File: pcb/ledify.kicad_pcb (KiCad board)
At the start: 4 copper layers, 35.5 x 52.5 mm, 74 parts, among them J1 Conn_01x01_Pin, J2 USB_C_Receptacle_USB2.0_16P, J3 Conn_01x01_Pin, J4 Conn_01x01_Pin, Q1 2N7002K, SW1 TS-1088-AR02016, SW2 TS-1088-AR02016, U1 ESP32-C6_C5364646, U2 USBLC6-2P6, U3 AP63203WU, U4 FUSB302BMPX, U5 W25Q128JVP, U6 LM61495QRPHRQ1, U7 BMI323, U8 BMP581, X1 XL2EL89COI-111YLC-40M, X2 Q13FC1350000400

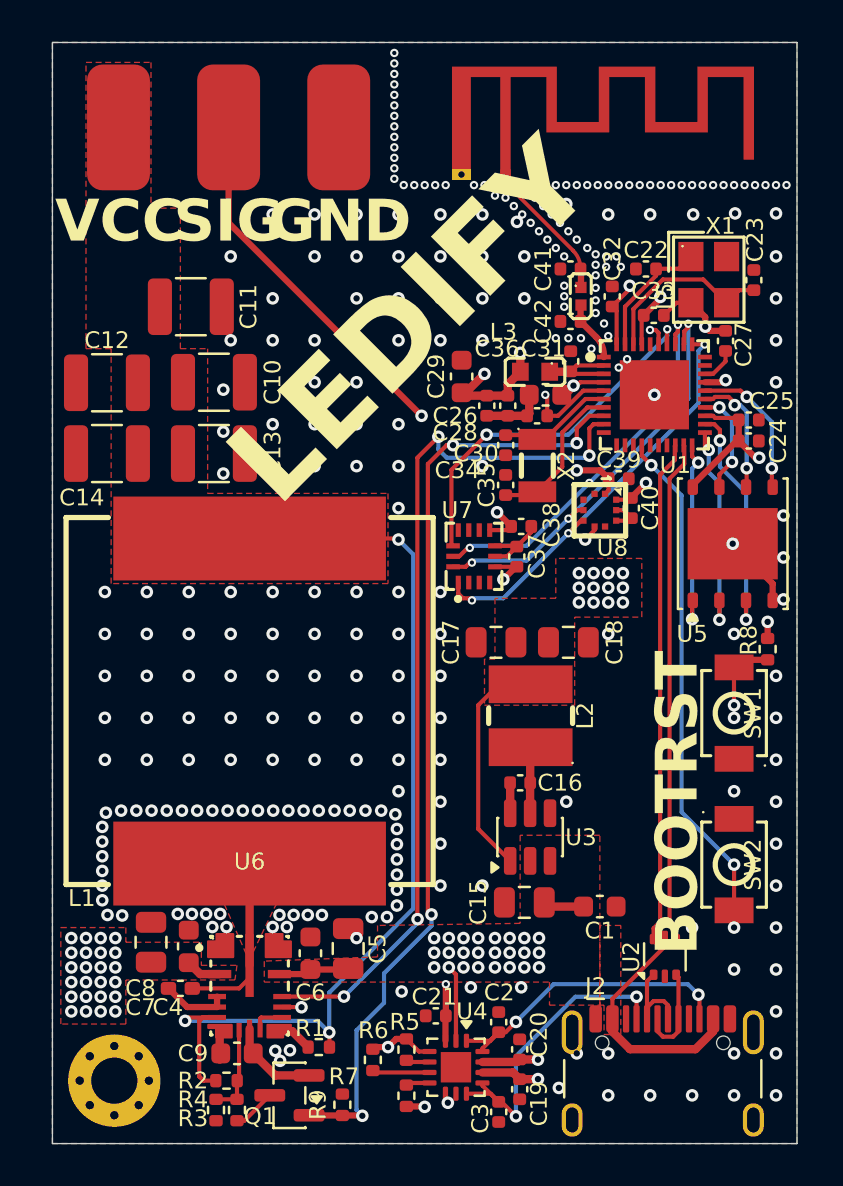
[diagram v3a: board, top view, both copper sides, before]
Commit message: blender render
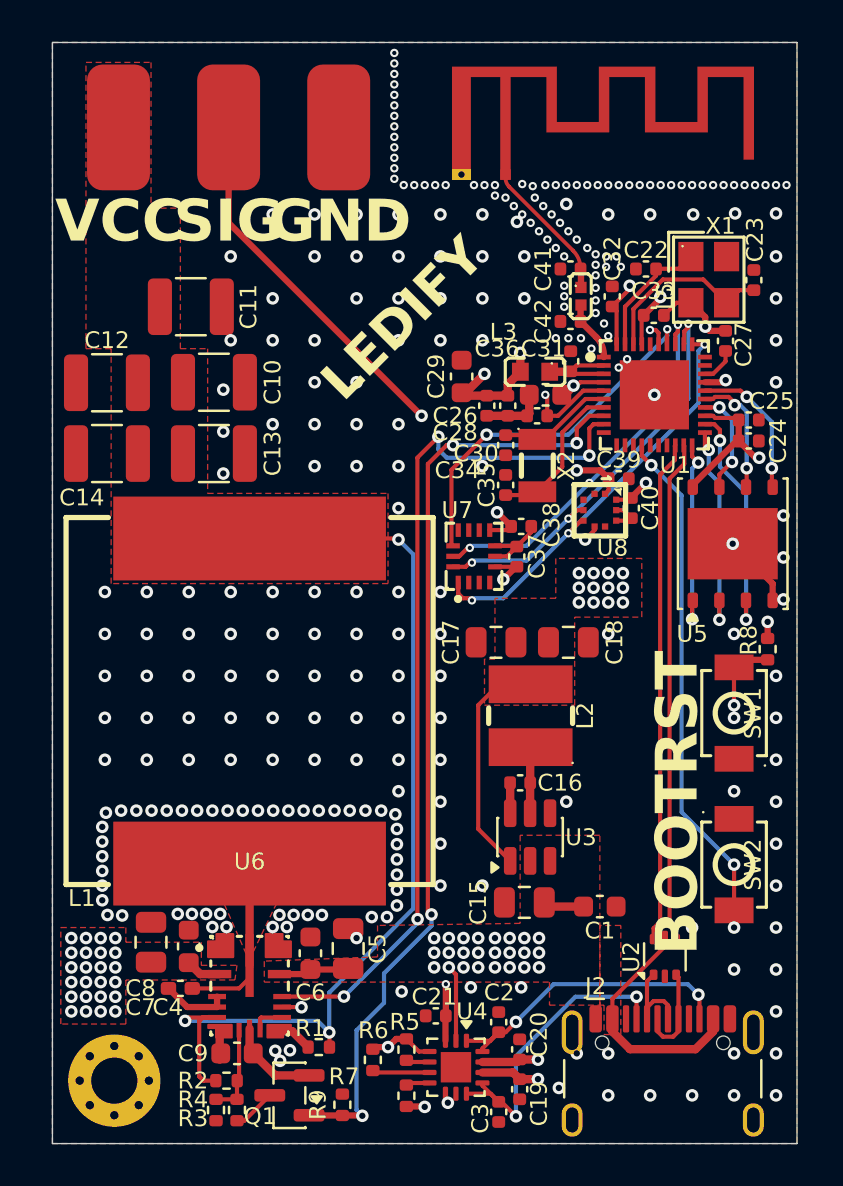
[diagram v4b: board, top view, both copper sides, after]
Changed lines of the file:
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@@
 	)
 	(gr_text "LEDIFY"
-		(at 73 50.55 45)
+		(at 71.75 49.5 45)
 		(layer "F.SilkS")
 		(effects
 			(font
-				(face "ByteBounce")
-				(size 4 4)
+				(face "Daydream")
+				(size 1.8 1.8)
 				(thickness 0.3)
 				(bold yes)
@@
 			(polygon
 				(pts
-					(xy 68.070439 53.027444) (xy 68.318445 52.779438) (xy 68.566277 53.027271) (xy 68.318445 53.275104)
-					(xy 68.070785 53.522764) (xy 67.822952 53.770597) (xy 67.575119 54.01843) (xy 67.327459 54.26609)
-					(xy 67.079626 54.513922) (xy 66.83283 54.267126) (xy 66.58586 54.020157) (xy 66.339064 53.77336)
-					(xy 66.092094 53.526391) (xy 65.845298 53.279594) (xy 65.598501 53.032798) (xy 65.845989 52.78531)
-					(xy 66.093476 52.537823) (xy 66.3401 52.784447) (xy 66.586724 53.031071) (xy 66.833348 53.277695)
-					(xy 67.079971 53.524318) (xy 67.326768 53.771115) (xy 67.574601 53.523282) (xy 67.822606 53.275277)
+					(xy 66.017696 52.450928) (xy 65.850681 52.617943) (xy 66.184789 52.952051) (xy 66.017696 53.119144)
+					(xy 66.518819 53.620267) (xy 66.351804 53.787282) (xy 67.192087 54.627564) (xy 67.359102 54.460549)
+					(xy 67.526117 54.627564) (xy 68.3664 53.787282) (xy 68.199385 53.620267) (xy 68.3664 53.453252)
+					(xy 68.027318 53.11417) (xy 67.860303 53.281185) (xy 67.69321 53.114092) (xy 67.359102 53.4482)
+					(xy 67.029968 53.119066) (xy 67.196983 52.952051) (xy 66.862875 52.617943) (xy 67.029968 52.45085)
+					(xy 66.523871 51.944753) (xy 66.356778 52.111846) (xy 66.189685 51.944753) (xy 65.850603 52.283835)
 				)
 			)
 			(polygon
 				(pts
-					(xy 69.80026 51.297623) (xy 70.048266 51.049617) (xy 70.296098 51.29745) (xy 70.048266 51.545283)
-					(xy 69.800606 51.792943) (xy 69.552773 52.040776) (xy 69.30494 52.288609) (xy 69.05728 52.536269)
-					(xy 68.809447 52.784101) (xy 68.562651 52.537305) (xy 68.315681 52.290336) (xy 68.068885 52.043539)
-					(xy 67.821915 51.79657) (xy 67.575119 51.549773) (xy 67.328322 51.302977) (xy 67.576155 51.055144)
-					(xy 67.823815 50.807484) (xy 68.071648 50.559651) (xy 68.319481 50.311818) (xy 68.567141 50.064158)
-					(xy 68.814974 49.816325) (xy 69.062806 50.064158) (xy 68.814801 50.312164) (xy 68.566968 50.559996)
-					(xy 68.318963 50.808002) (xy 68.07113 51.055835) (xy 68.309637 51.294341) (xy 68.556779 51.047199)
-					(xy 68.803921 50.800057) (xy 69.051753 51.04789) (xy 68.804611 51.295032) (xy 68.557469 51.542174)
-					(xy 68.806857 51.791561) (xy 69.056589 52.041294) (xy 69.304422 51.793461) (xy 69.552427 51.545456)
+					(xy 67.353195 51.115429) (xy 67.18618 51.282444) (xy 67.520288 51.616552) (xy 67.353195 51.783644)
+					(xy 67.854318 52.284767) (xy 67.687303 52.451783) (xy 68.527586 53.292065) (xy 68.694601 53.12505)
+					(xy 68.861616 53.292065) (xy 70.036007 52.117675) (xy 69.868992 51.95066) (xy 70.036007 51.783644)
+					(xy 69.696925 51.444563) (xy 68.861694 52.279794) (xy 68.699575 52.117675) (xy 69.200698 51.616552)
+					(xy 69.033683 51.449536) (xy 69.200776 51.282444) (xy 68.861694 50.943362) (xy 68.360493 51.444563)
+					(xy 68.198374 51.282444) (xy 68.86659 50.614228) (xy 68.699575 50.447213) (xy 68.866668 50.28012)
+					(xy 68.527586 49.941038) (xy 68.360493 50.108131) (xy 68.1934 49.941038) (xy 67.186102 50.948336)
 				)
 			)
 			(polygon
 				(pts
-					(xy 71.031134 48.583897) (xy 71.27983 48.832593) (xy 71.528527 49.08129) (xy 71.777223 49.329986)
-					(xy 71.529736 49.577473) (xy 71.772905 49.820643) (xy 71.526109 50.06744) (xy 71.279485 50.314063)
-					(xy 71.032689 50.56086) (xy 70.786065 50.807484) (xy 70.539268 51.05428) (xy 70.292472 50.807484)
-					(xy 70.045502 50.560515) (xy 69.798706 50.313718) (xy 69.551737 50.066749) (xy 69.30494 49.819952)
-					(xy 69.058143 49.573156) (xy 69.30494 49.326359) (xy 69.305285 49.326014) (xy 69.800951 49.326014)
-					(xy 70.047229 49.572292) (xy 70.293681 49.818743) (xy 70.539959 50.065022) (xy 70.78641 50.311473)
-					(xy 71.031998 50.065885) (xy 71.277585 49.820298) (xy 71.031134 49.573847) (xy 70.784856 49.327568)
-					(xy 70.538405 49.081117) (xy 70.292126 48.834839) (xy 70.046539 49.080426) (xy 69.800951 49.326014)
-					(xy 69.305285 49.326014) (xy 69.551564 49.079735) (xy 69.79836 48.832939) (xy 70.044984 48.586315)
-					(xy 70.291781 48.339518) (xy 70.53495 48.582688) (xy 70.782438 48.335201)
+					(xy 70.865331 48.605539) (xy 71.032346 48.438524) (xy 72.039644 49.445821) (xy 71.872629 49.612836)
+					(xy 72.039722 49.779929) (xy 71.872629 49.947022) (xy 72.039644 50.114037) (xy 70.698238 51.455443)
+					(xy 70.030023 50.787227) (xy 69.863007 50.954242) (xy 68.688695 49.779929) (xy 68.85571 49.612914)
+					(xy 68.855632 49.612836) (xy 69.867981 49.612836) (xy 70.364208 50.109063) (xy 70.531223 49.942048)
+					(xy 70.698238 50.109063) (xy 70.860357 49.946944) (xy 70.693342 49.779929) (xy 70.860357 49.612914)
+					(xy 70.531223 49.28378) (xy 70.364208 49.450795) (xy 70.197115 49.283702) (xy 69.867981 49.612836)
+					(xy 68.855632 49.612836) (xy 68.688617 49.445821) (xy 69.695915 48.438524) (xy 69.863007 48.605616)
+					(xy 70.197115 48.271508) (xy 70.364131 48.438524) (xy 70.531223 48.271431)
 				)
 			)
 			(polygon
 				(pts
-					(xy 73.015178 48.57837) (xy 72.766482 48.827067) (xy 72.517785 49.075763) (xy 72.269089 49.324459)
-					(xy 72.021256 49.076627) (xy 72.266844 48.831039) (xy 72.020393 48.584588) (xy 71.774114 48.338309)
-					(xy 71.527663 48.091858) (xy 71.281385 47.84558) (xy 71.035797 48.091167) (xy 70.787964 47.843335)
-					(xy 71.036661 47.594638) (xy 71.285357 47.345942) (xy 71.534053 47.097246) (xy 71.78275 46.848549)
-					(xy 72.030582 47.096382) (xy 71.77636 47.350605) (xy 72.022638 47.596884) (xy 72.269089 47.843335)
-					(xy 72.515368 48.089613) (xy 72.761819 48.336064) (xy 73.016042 48.081841) (xy 73.263874 48.329674)
+					(xy 70.860202 47.608422) (xy 70.693187 47.775437) (xy 72.368701 49.450951) (xy 72.535716 49.283936)
+					(xy 72.702731 49.450951) (xy 73.208905 48.944776) (xy 73.04189 48.777761) (xy 73.208905 48.610746)
+					(xy 72.535716 47.937556) (xy 72.368701 48.104571) (xy 71.366377 47.102247) (xy 71.199284 47.26934)
+					(xy 71.032191 47.102247) (xy 70.693109 47.441329)
 				)
 			)
 			(polygon
 				(pts
-					(xy 73.751768 47.84178) (xy 73.504281 48.089268) (xy 73.257484 47.842471) (xy 73.010515 47.595502)
-					(xy 72.763718 47.348705) (xy 72.516749 47.101736) (xy 72.269953 46.85494) (xy 72.023156 46.608143)
-					(xy 72.270989 46.36031) (xy 72.518649 46.11265) (xy 72.766482 45.864817) (xy 73.014315 45.616985)
-					(xy 73.261975 45.369324) (xy 73.509807 45.121492) (xy 73.75764 45.369324) (xy 73.509635 45.61733)
-					(xy 73.261802 45.865163) (xy 73.013796 46.113168) (xy 72.765964 46.361001) (xy 73.00447 46.599508)
-					(xy 73.251612 46.352366) (xy 73.498754 46.105224) (xy 73.746587 46.353057) (xy 73.499445 46.600198)
-					(xy 73.252303 46.84734) (xy 73.501172 47.096209) (xy 73.750387 47.345424) (xy 73.999256 47.594293)
+					(xy 72.029541 46.439083) (xy 71.862448 46.606176) (xy 72.363571 47.107299) (xy 72.196556 47.274314)
+					(xy 73.370947 48.448705) (xy 73.537962 48.281689) (xy 73.704977 48.448705) (xy 74.044059 48.109623)
+					(xy 73.877044 47.942608) (xy 74.044136 47.775515) (xy 73.542936 47.274314) (xy 74.044059 46.773191)
+					(xy 73.877044 46.606176) (xy 74.044136 46.439083) (xy 73.705055 46.100001) (xy 73.203854 46.601202)
+					(xy 73.041735 46.439083) (xy 73.542936 45.937882) (xy 73.375921 45.770867) (xy 73.542936 45.603852)
+					(xy 73.203854 45.26477) (xy 73.036839 45.431785) (xy 72.869746 45.264692) (xy 71.862448 46.27199)
 				)
 			)
 			(polygon
 				(pts
-					(xy 75.978982 45.614567) (xy 75.731494 45.862054) (xy 75.484698 45.615257) (xy 75.237729 45.368288)
-					(xy 74.983506 45.622511) (xy 74.736709 45.375715) (xy 74.49354 45.618884) (xy 74.24657 45.371915)
-					(xy 73.999774 45.125118) (xy 73.752977 44.878322) (xy 74.000465 44.630835) (xy 74.247952 44.383347)
-					(xy 74.494748 44.630144) (xy 74.741545 44.87694) (xy 74.988514 45.12391) (xy 75.237211 44.875213)
-					(xy 75.485907 44.626517) (xy 75.238938 44.379548) (xy 74.992141 44.132751) (xy 74.745345 43.885955)
-					(xy 74.989723 43.641576) (xy 75.234102 43.397197) (xy 75.480898 43.643994) (xy 75.727695 43.89079)
-					(xy 75.974664 44.13776) (xy 75.731494 44.380929) (xy 75.978291 44.627726) (xy 75.732703 44.873313)
-					(xy 75.979673 45.120283) (xy 76.226469 45.367079)
+					(xy 74.534768 43.933856) (xy 74.367753 44.100871) (xy 74.701861 44.434979) (xy 74.539742 44.597098)
+					(xy 74.372649 44.430005) (xy 74.205634 44.59702) (xy 74.038619 44.430005) (xy 73.532444 44.93618)
+					(xy 73.699459 45.103195) (xy 73.532444 45.27021) (xy 73.871526 45.609292) (xy 74.038541 45.442277)
+					(xy 74.205634 45.60937) (xy 74.372726 45.442277) (xy 74.539742 45.609292) (xy 74.706757 45.442277)
+					(xy 74.87385 45.60937) (xy 75.040942 45.442277) (xy 75.202984 45.604318) (xy 75.035891 45.771411)
+					(xy 75.542065 46.277586) (xy 75.709158 46.110493) (xy 75.876173 46.277508) (xy 76.215255 45.938426)
+					(xy 76.04824 45.771411) (xy 76.215255 45.604396) (xy 75.881147 45.270288) (xy 76.04824 45.103195)
+					(xy 75.714132 44.769087) (xy 75.881147 44.602072) (xy 75.547039 44.267964) (xy 75.714132 44.100871)
+					(xy 75.040942 43.427681) (xy 74.87385 43.594774) (xy 74.706757 43.427681) (xy 74.367675 43.766763)
 				)
 			)

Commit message: cool font thing
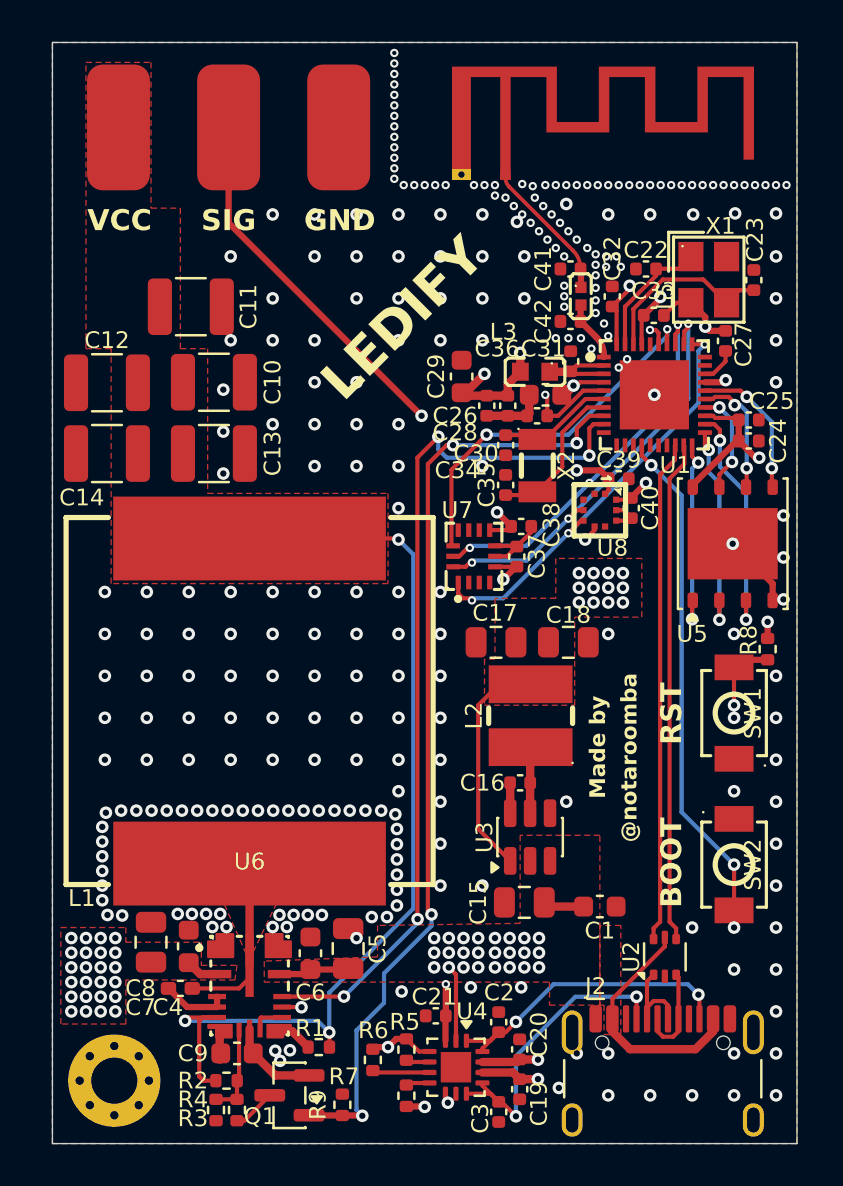
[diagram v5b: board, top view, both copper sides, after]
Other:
- board text added: "@notaroomba"
- board text added: "Made by"
